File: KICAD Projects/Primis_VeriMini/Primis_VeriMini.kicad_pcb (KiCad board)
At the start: 2 copper layers, 50 x 26 mm, 33 parts, among them J1 USB-05, J2 Conn_ARM_SWD_TagConnect_TC203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, U1 nRF52833_QDxx, Y2 Crystal_GND24

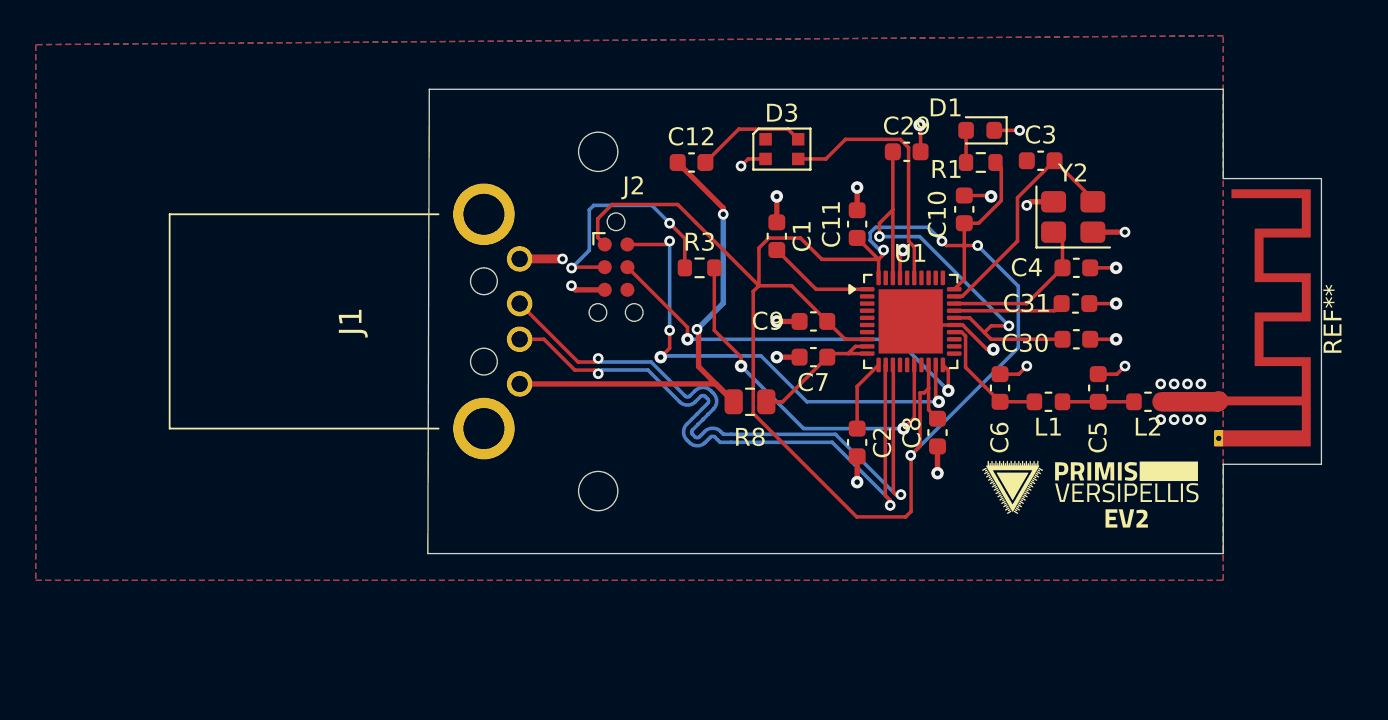
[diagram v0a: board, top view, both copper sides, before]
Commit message: CleanUp
-Added Locus EV1 STEP and STL files
-Added Locus PCB picture
-Added very early work on PI3 carrier board
-Added nearly complete VeriMini kicad project
-Added extra details to README
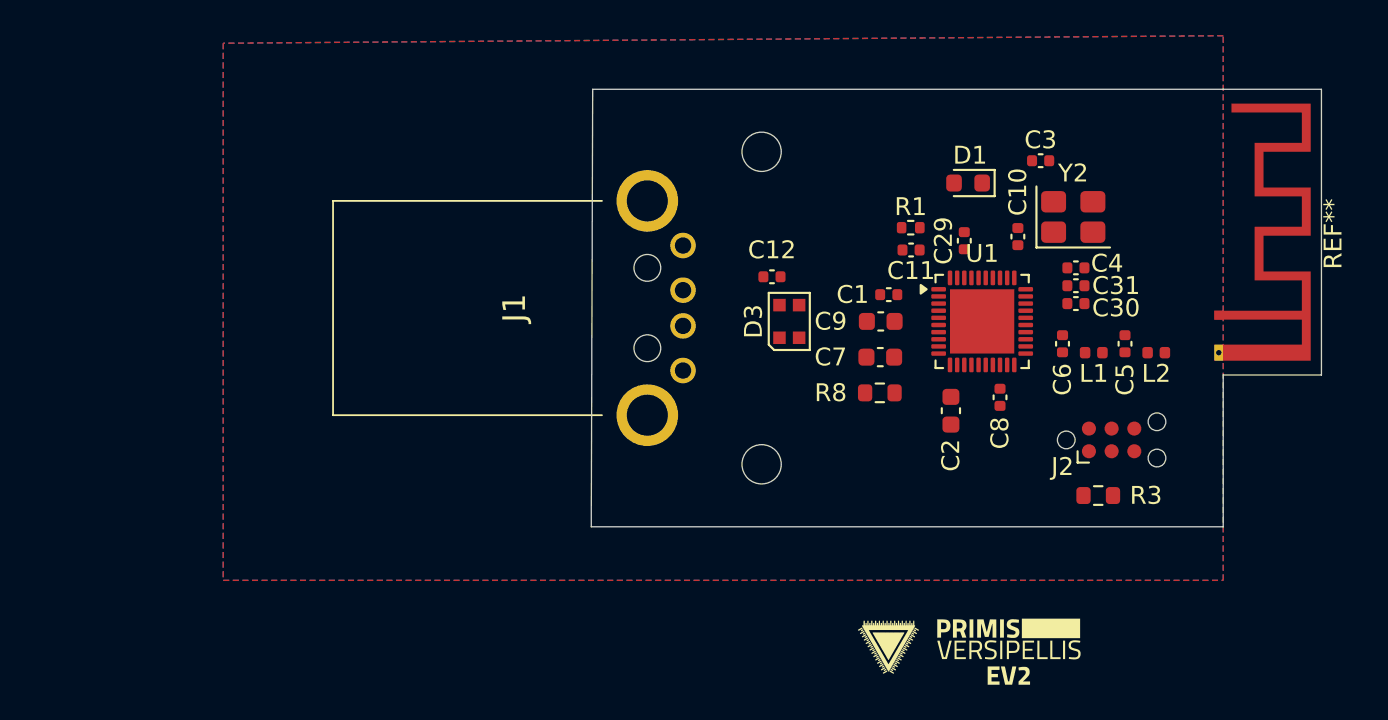
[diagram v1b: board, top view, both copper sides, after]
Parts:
- C1, C10, C11, C12, C29, C3, C30, C31, C4, C5, C6, C8: footprint Capacitor_SMD:C_0603_1608Metric -> Capacitor_SMD:C_0402_1005Metric
- L1, L2: footprint Inductor_SMD:L_0603_1608Metric -> Inductor_SMD:L_0402_1005Metric
- R1: footprint Resistor_SMD:R_0603_1608Metric -> Resistor_SMD:R_0402_1005Metric
- R8: footprint Resistor_SMD:R_0805_2012Metric -> Resistor_SMD:R_0603_1608Metric
- moved J2 29.4 mm to (162.8, 76.1), turned to 0 degrees
- moved R3 25.7 mm to (162.0, 79.2), turned to 180 degrees
- moved G*** 11.3 mm to (150.2, 87.8)
- moved G*** 11.0 mm to (157.0, 88.0)
- moved D3 9.66 mm to (144.7, 69.5), turned to 90 degrees
- moved H1 9.27 mm to (143.2, 77.5)
- moved J1 9.18 mm to (138.8, 65.2)
- moved H2 9.15 mm to (143.2, 60.0)
- moved C12 7.83 mm to (143.7, 67.0)
- moved R8 7.29 mm to (149.8, 73.5)
- moved C1 7.07 mm to (150.3, 68.0), turned to 0 degrees
- moved C29 5.93 mm to (154.5, 65.0), turned to 90 degrees
- moved C2 5.54 mm to (153.8, 74.5)
- moved R1 5.36 mm to (151.5, 64.2)
- moved REF** 4.80 mm to (168.8, 69.2)
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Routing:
- net VDD_nRF: track 94.3 -> 0.00 mm, vias 4 -> 0
- net D+: track 37.3 -> 0.00 mm, vias 2 -> 0
- net D-: track 36.7 -> 0.00 mm, vias 2 -> 0
- net GND: track 36.7 -> 0.00 mm, vias 29 -> 0
- net VBUS: track 28.3 -> 0.00 mm, vias 2 -> 0
- net Net-(J2-SWDIO): track 27.9 -> 0.00 mm, vias 4 -> 0
- net DEC4_6: track 26.3 -> 0.00 mm, vias 2 -> 0
- net Net-(J2-SWCLK): track 22.8 -> 0.00 mm, vias 2 -> 0
- net Net-(U1-P0.18/~{RESET}): track 20.5 -> 0.00 mm, vias 2 -> 0
- net Net-(D3-DIN): track 14.3 -> 0.00 mm
- net Net-(J2-~{RESET}): track 13.4 -> 0.00 mm, vias 2 -> 0
- net Net-(U1-XC2): track 13.4 -> 0.00 mm
- net Net-(U1-XC1): track 9.10 -> 0.00 mm
- net Net-(U1-VBUS): track 8.00 -> 0.00 mm
- net Net-(U1-ANT): track 7.13 -> 0.00 mm
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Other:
- board size 50 x 26 mm -> 40.9 x 24.5 mm
